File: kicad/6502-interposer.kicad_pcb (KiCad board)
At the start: 2 copper layers, 68.5 x 44.4 mm, 6 parts, among them J1 LogicAnalyzer #1, J2 LogicAnalyzer #2, J3 Conn_02x09_Odd_Even, U1 65CE02

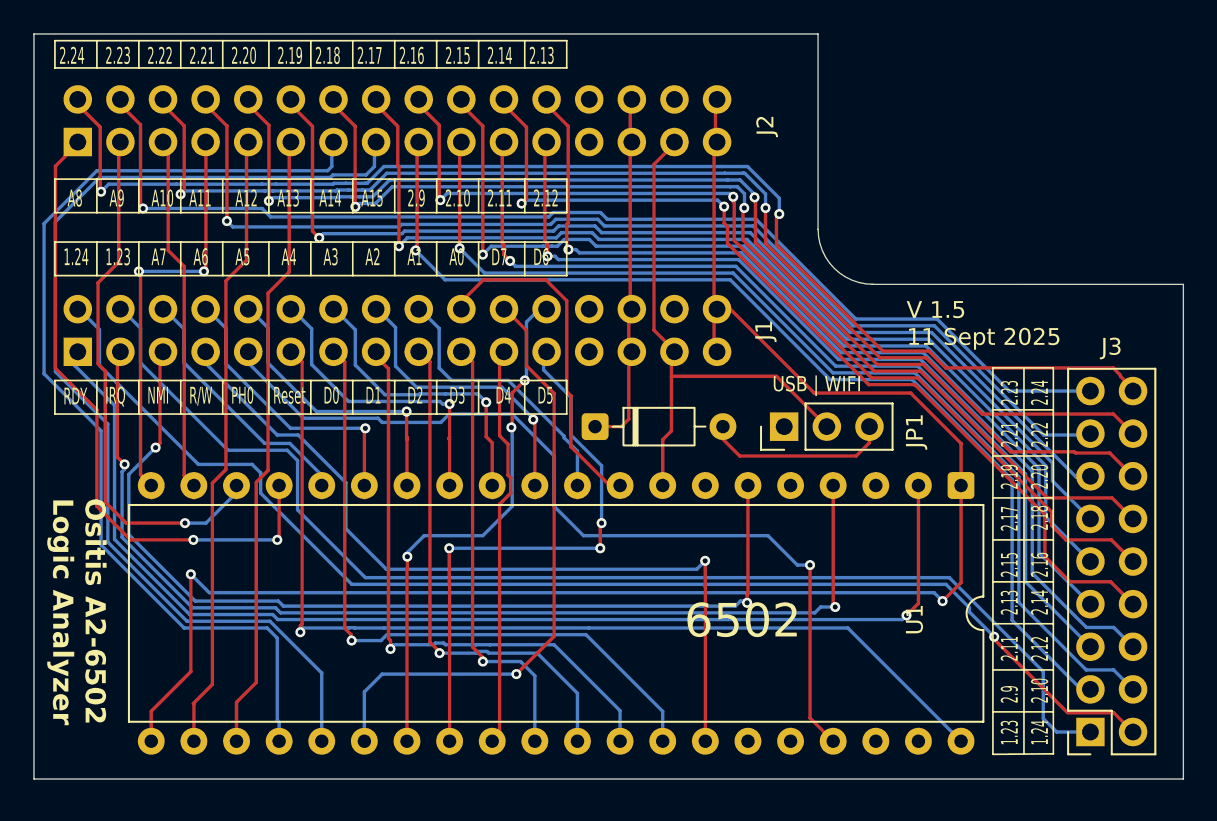
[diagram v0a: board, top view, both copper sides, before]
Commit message: updates for v1.5
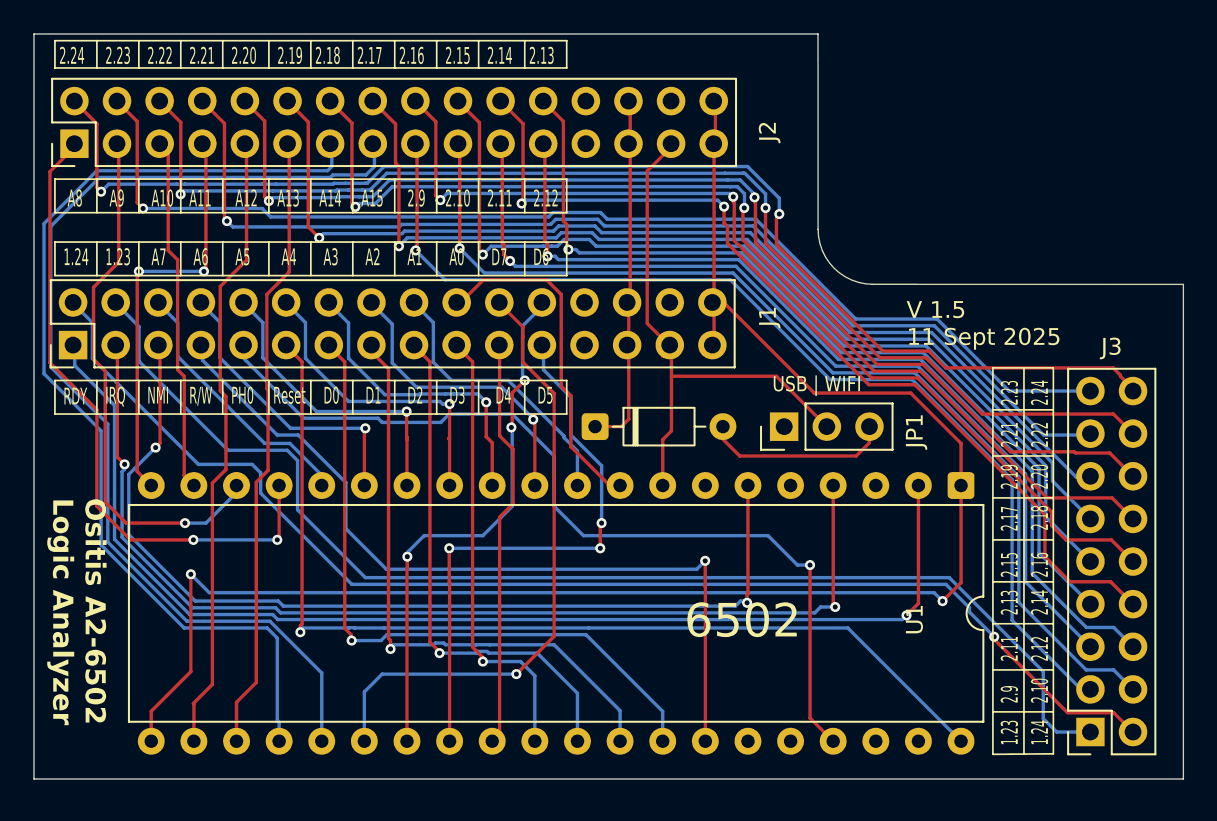
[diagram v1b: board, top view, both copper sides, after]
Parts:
- J1, J2: moved to F.Cu
- moved J1 2.95 mm to (47.6, 53.6), turned to 90 degrees
- moved J2 2.45 mm to (47.7, 41.6), turned to 90 degrees
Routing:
- net /A11: track 25.5 -> 24.6 mm
